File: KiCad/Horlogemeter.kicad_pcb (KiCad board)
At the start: 2 copper layers, 71 x 53 mm, 48 parts, among them J1 Serial header, J10 I2c spare, J2 AVR-ISP-6, J3 Piezo microphone, J4 12v input, J5 Headphones, J6 Gain pot 10k, J7 RTC connector board, J8 External LED, J9 I2c display connector, Q1 BC327, U1 ATmega328P-PU, U2 TL072, U3 OPA37GP, U4 L7805, Y1 16Mhz

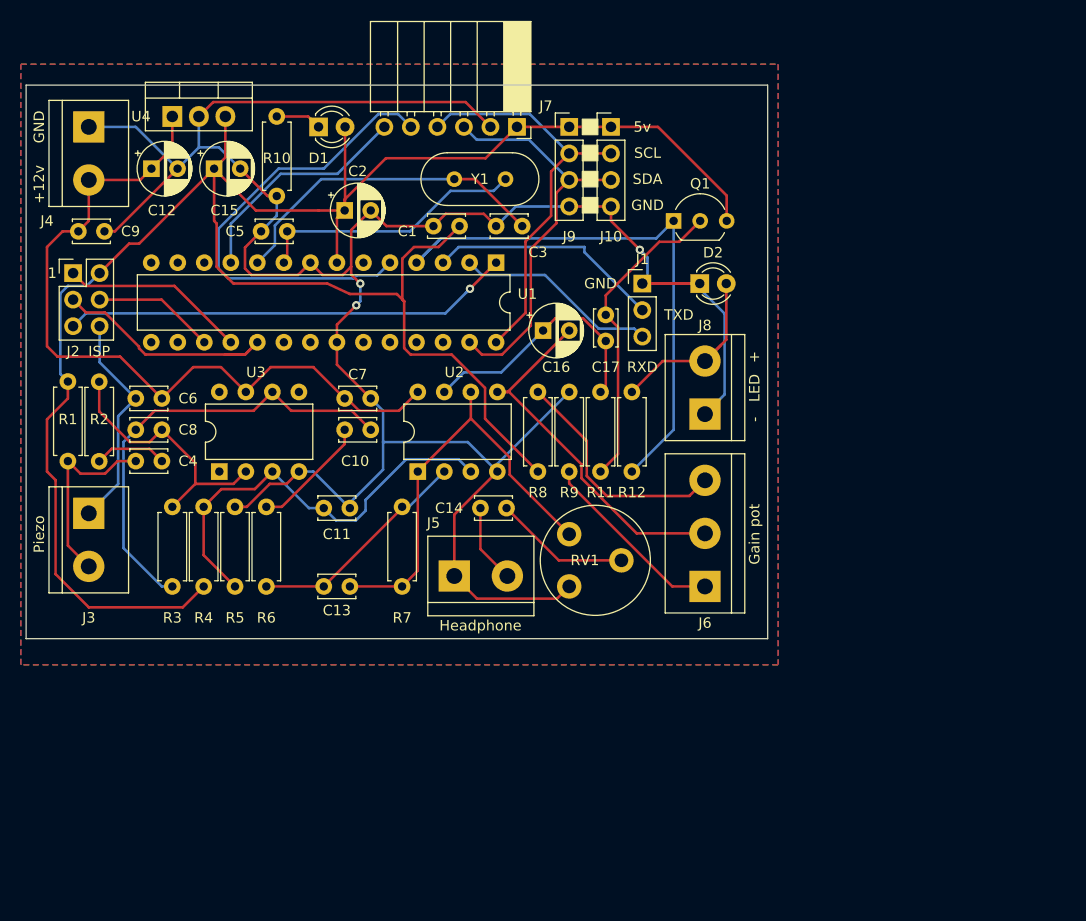
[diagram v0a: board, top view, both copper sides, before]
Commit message: Created new PCB with Gerbers
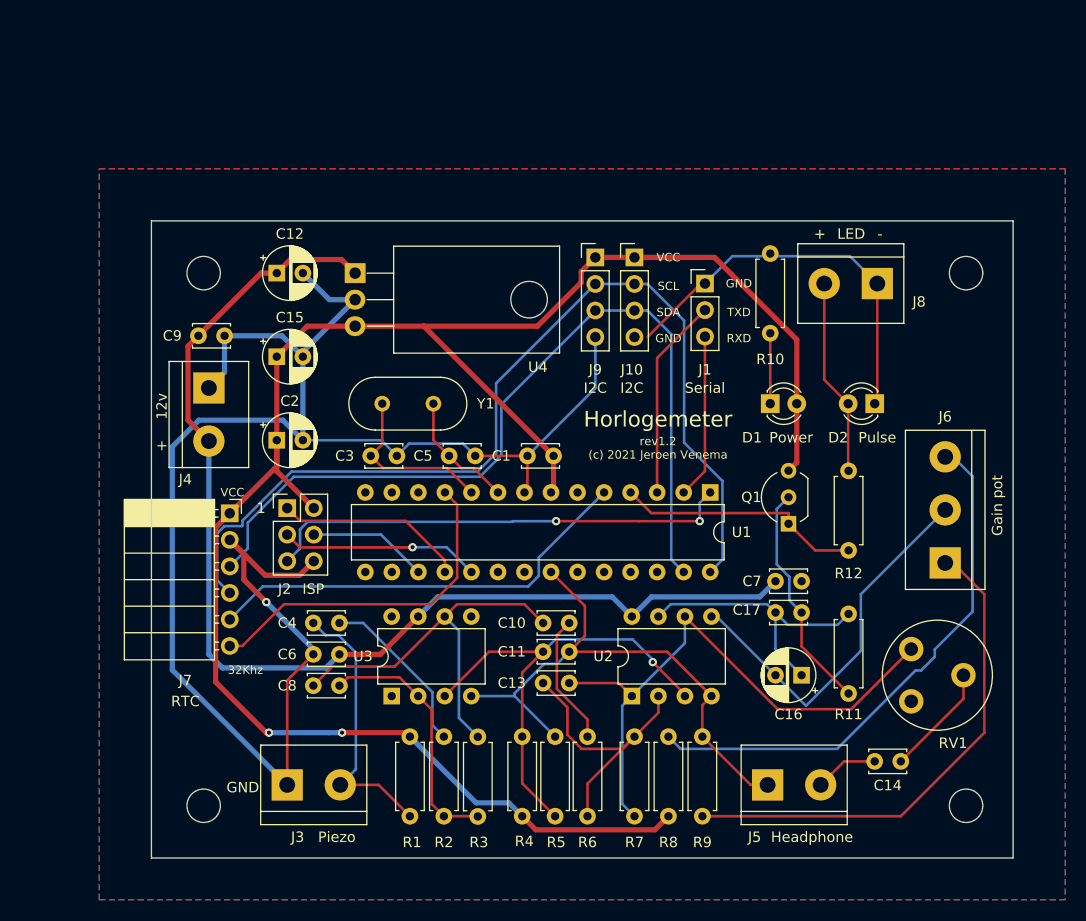
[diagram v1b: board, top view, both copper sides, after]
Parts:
- added REF**: MountingHole_3.2mm_M3, MountingHole:MountingHole_3.2mm_M3, F.Cu at (163.0, 80.0)
- added REF**: MountingHole_3.2mm_M3, MountingHole:MountingHole_3.2mm_M3, F.Cu at (163.0, 131.0)
- added REF**: MountingHole_3.2mm_M3, MountingHole:MountingHole_3.2mm_M3, F.Cu at (90.0, 131.0)
- added REF**: MountingHole_3.2mm_M3, MountingHole:MountingHole_3.2mm_M3, F.Cu at (90.0, 80.0)
- U4: footprint Package_TO_SOT_THT:TO-220-3_Vertical -> Package_TO_SOT_THT:TO-220-3_Horizontal_TabDown
- moved R2 53.1 mm to (113.0, 132.0), turned to 90 degrees
- moved R10 51.6 mm to (144.2, 85.8), turned to 90 degrees
- moved D1 50.7 mm to (144.2, 92.5)
- moved R1 47.2 mm to (109.8, 132.0)
- moved J7 46.1 mm to (92.5, 103.0), turned to 0 degrees
- moved C14 44.9 mm to (156.8, 126.8)
- moved C7 44.8 mm to (144.8, 109.5)
- moved C16 41.2 mm to (147.2, 118.5), turned to 180 degrees
- moved R6 37.8 mm to (126.8, 132.0)
- moved R5 37.7 mm to (123.7, 132.0)
- moved R4 37.6 mm to (120.5, 132.0)
- moved J5 36.1 mm to (144.0, 129.0)
- moved R9 35.4 mm to (137.8, 132.0)
- moved R8 35.3 mm to (134.5, 132.0)
- moved RV1 34.5 mm to (157.8, 121.0)
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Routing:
- net /SCL: track 39.7 -> 92.5 mm
- net /SDA: track 39.2 -> 80.9 mm
- net +12V: track 74.0 -> 110.1 mm
- net Net-(Q1-Pad1): track 55.2 -> 23.8 mm
- net Net-(J6-Pad1): track 18.2 -> 48.6 mm
- net Net-(J6-Pad3): track 22.7 -> 51.8 mm
- net VCC: track 206.4 -> 182.9 mm, vias 0 -> 2
- net Net-(C3-Pad1): track 31.6 -> 16.5 mm
- net Net-(C13-Pad1): track 41.3 -> 56.3 mm
- net Net-(C5-Pad1): track 26.1 -> 11.8 mm
- net /32Khz: track 22.3 -> 33.1 mm
- net Net-(C4-Pad2): track 6.99 -> 16.4 mm
- net Net-(C4-Pad1): track 18.4 -> 26.4 mm
- net Net-(C17-Pad2): track 30.1 -> 22.1 mm
- net Net-(C13-Pad2): track 21.7 -> 27.7 mm
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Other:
- board size 71 x 53 mm -> 82.5 x 61 mm
- board text added: "12v"
- board text added: "32Khz"
- board text added: "Horlogemeter"
- board text added: "I2C"
- board text added: "Power"
- board text added: "Pulse"
- board text added: "RTC"
- board text added: "Serial"
- board text added: "VCC"
- board text added: "rev1.2 (c) 2021 Jeroen Venema"
- board text removed: "+12v"
- board text removed: "5v"
- board text removed: "Horlogemeter rev1.1 (c) 2021 Jeroen Venema"
